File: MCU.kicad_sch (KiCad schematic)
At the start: 36 parts

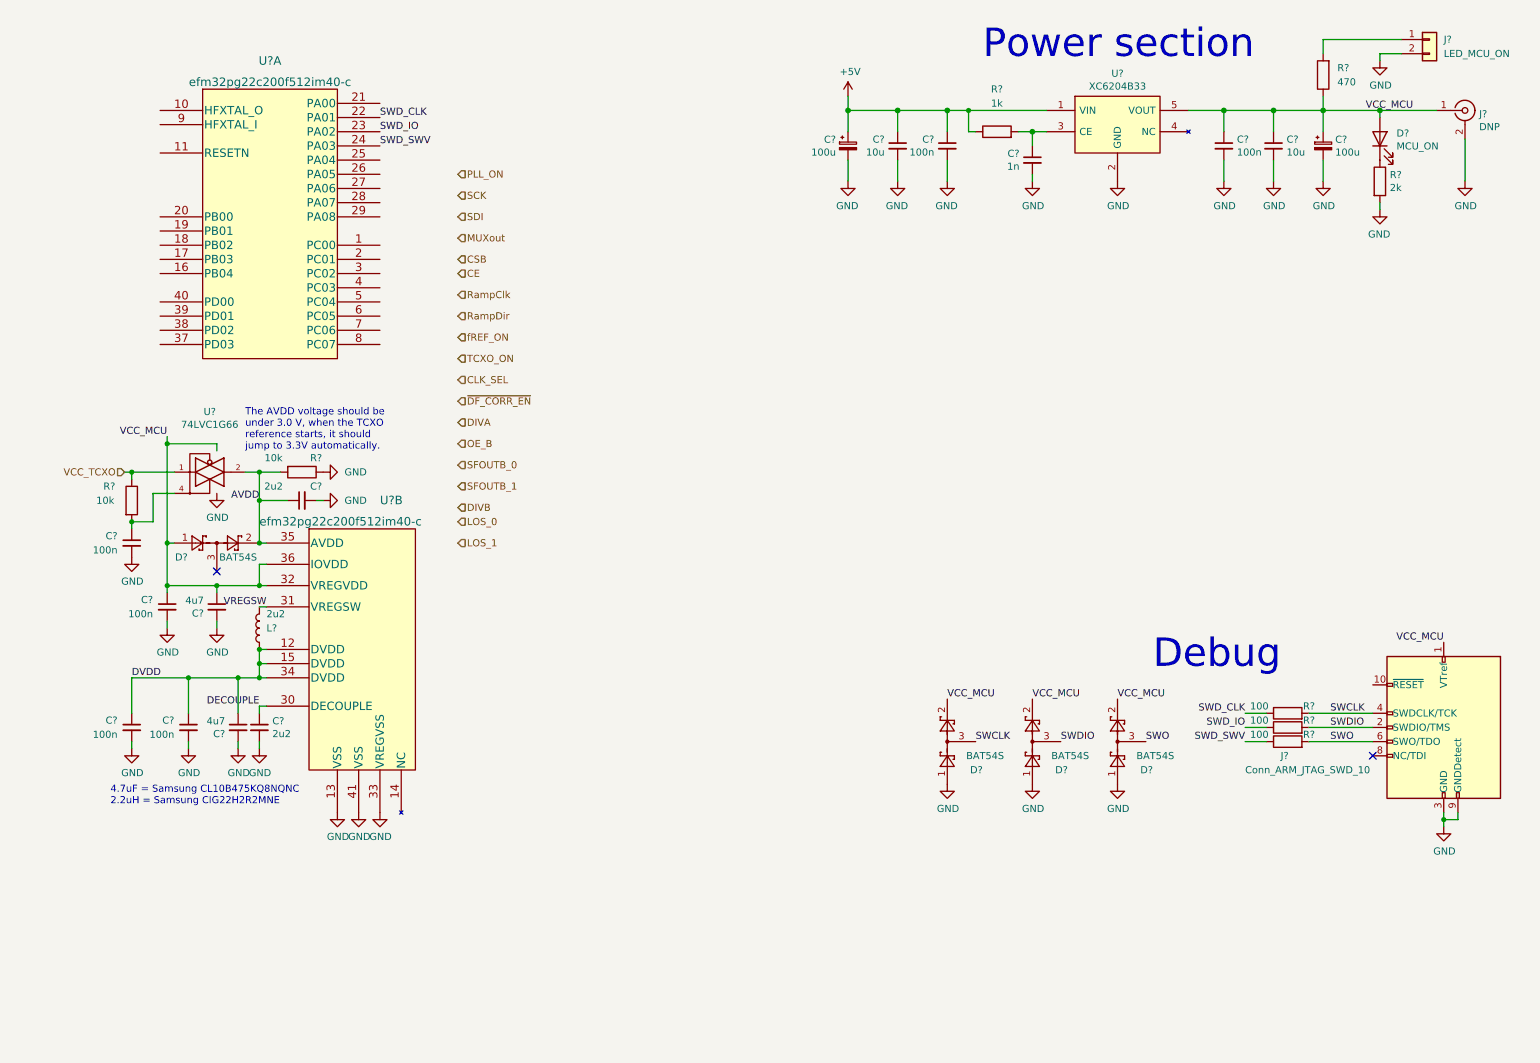
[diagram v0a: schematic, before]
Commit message: Updates to schematic
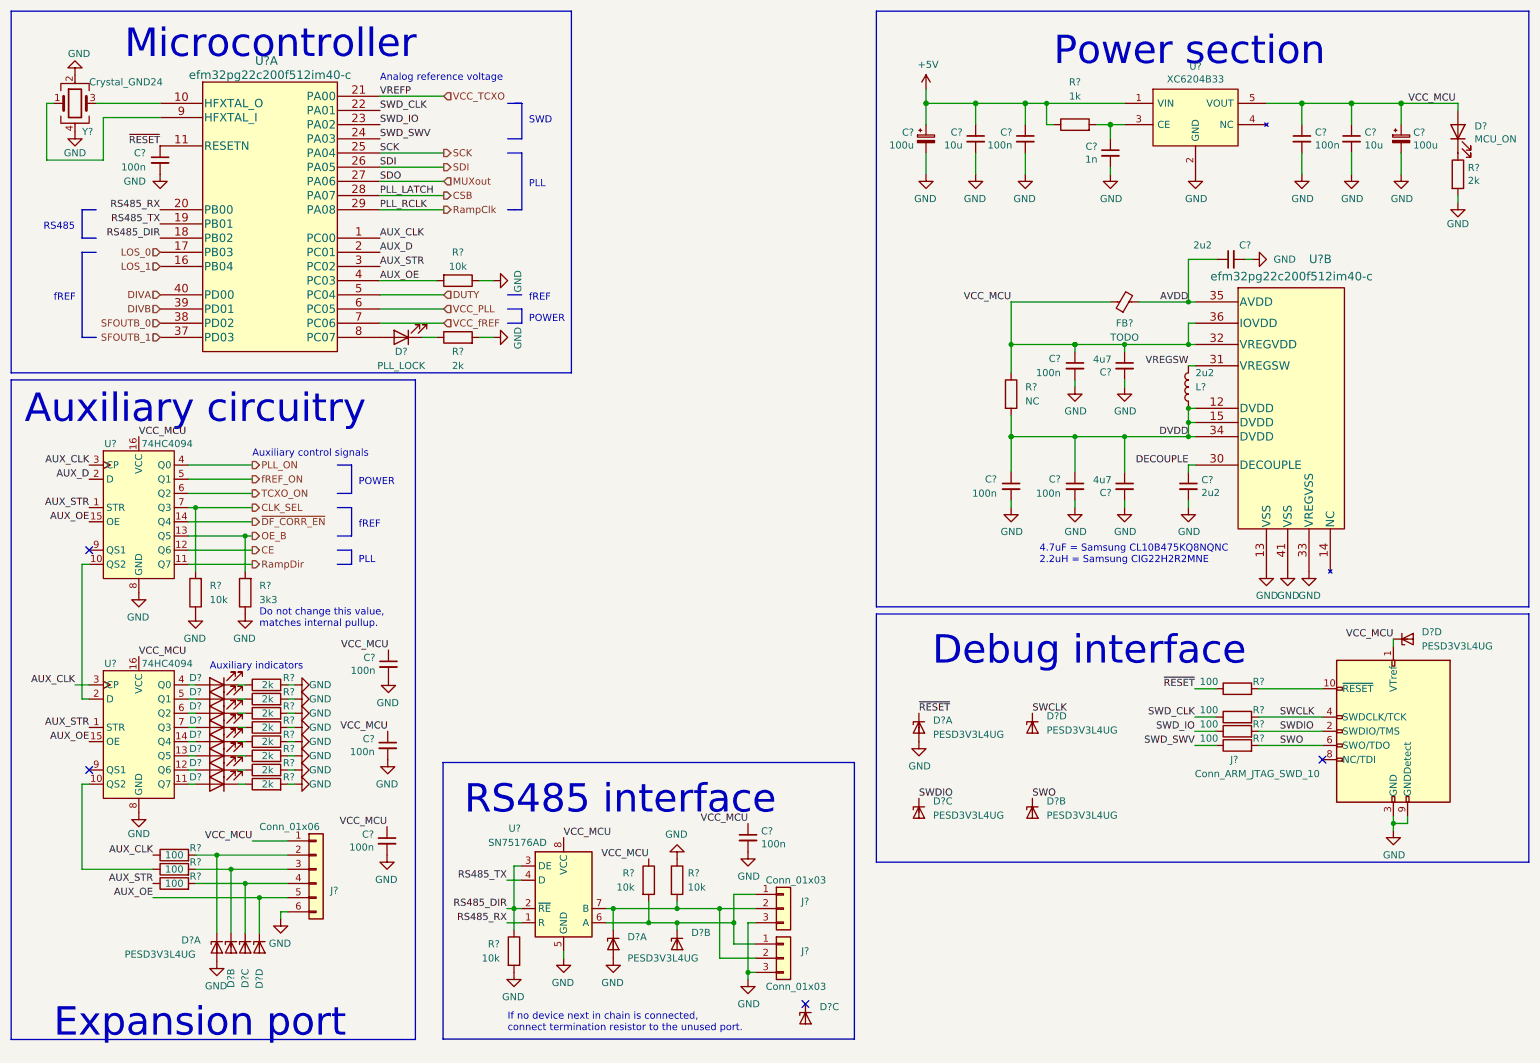
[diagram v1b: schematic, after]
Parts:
- removed C?: 100n, Capacitor_SMD:C_0603_1608Metric_Pad1.08x0.95mm_HandSolder, symbol Device:C_Small
- removed D? (x4): BAT54S, Package_TO_SOT_SMD:SOT-23, symbol Diode:BAT54S
- removed J?: LED_MCU_ON, symbol Connector_Generic:Conn_01x02
- removed J?: DNP, Connector_Coaxial:U.FL_Molex_MCRF_73412-0110_Vertical, symbol Connector:Conn_Coaxial
- removed R?: 470, Resistor_SMD:R_0603_1608Metric_Pad0.98x0.95mm_HandSolder, symbol Device:R
- removed R? (x2): 10k, Resistor_SMD:R_0603_1608Metric_Pad0.98x0.95mm_HandSolder, symbol Device:R
- removed U?: 74LVC1G66, Package_TO_SOT_SMD:SOT-353_SC-70-5_Handsoldering, symbol 74xGxx:74LVC1G66
- added C? (x5): 100n, Capacitor_SMD:C_0603_1608Metric_Pad1.08x0.95mm_HandSolder, symbol Device:C_Small
- added D?: PLL_LOCK, LED_SMD:LED_0603_1608Metric_Pad1.05x0.95mm_HandSolder, symbol Device:LED
- added D? (x8): (no value), LED_SMD:LED_0603_1608Metric_Pad1.05x0.95mm_HandSolder, symbol Device:LED
- added D? (x12): PESD3V3L4UG, Package_TO_SOT_SMD:SOT-353_SC-70-5, symbol Power_Protection:PESD3V3L4UG
- added FB?: TODO, symbol Device:FerriteBead_Small
- added J? (x2): Conn_01x03, symbol Connector_Generic:Conn_01x03
- added J?: Conn_01x06, symbol Connector_Generic:Conn_01x06
- added R? (x4): 100, Resistor_SMD:R_0603_1608Metric_Pad0.98x0.95mm_HandSolder, symbol Device:R
- added R? (x9): 2k, Resistor_SMD:R_0603_1608Metric_Pad0.98x0.95mm_HandSolder, symbol Device:R
- added R? (x5): 10k, Resistor_SMD:R_0603_1608Metric_Pad0.98x0.95mm_HandSolder, symbol Device:R
- added R?: 3k3, Resistor_SMD:R_0603_1608Metric_Pad0.98x0.95mm_HandSolder, symbol Device:R
- added R?: NC, Resistor_SMD:R_0603_1608Metric_Pad0.98x0.95mm_HandSolder, symbol Device:R
- added U? (x2): 74HC4094, Package_SO:SO-16_3.9x9.9mm_P1.27mm, symbol petr:74HC4094
- added U?: SN75176AD, Package_SO:SOIC-8_3.9x4.9mm_P1.27mm, symbol Interface_UART:SN75176AD
- added Y?: Crystal_GND24, symbol Device:Crystal_GND24
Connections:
- net AVDD: now also FB?.2
- net CE: now also U?.12 (Q6)
- net CLK_SEL: now also R?.2, U?.7 (Q3)
- net CSB: now also U?.28 (PA07)
- net DIVA: now also U?.40 (PD00)
- net DIVB: now also U?.39 (PD01)
- net GND: now also C?.2, C?.2, C?.2, C?.2, C?.2, D?.2 (A), D?.2 (A), D?.2 (A), J?.3 (Pin_3), J?.3 (Pin_3), J?.6 (Pin_6), R?.1, R?.1, R?.1, R?.1, R?.2, R?.2, R?.2, R?.2, R?.2, R?.2, R?.2, R?.2, R?.2, R?.2, U?.5 (GND), U?.8 (GND), U?.8 (GND), Y?.2, Y?.4
- net LOS_0: now also U?.17 (PB03)
- net LOS_1: now also U?.16 (PB04)
- net MUXout: now also U?.27 (PA06)
- net OE_B: now also R?.2, U?.13 (Q5)
- net PLL_ON: now also U?.4 (Q0)
- net RampClk: now also U?.29 (PA08)
- net RampDir: now also U?.11 (Q7)
- net SCK: now also U?.25 (PA04)
- net SDI: now also U?.26 (PA05)
- net SFOUTB_0: now also U?.38 (PD02)
- net SFOUTB_1: now also U?.37 (PD03)
- net SWCLK: now also D?.5 (K4)
- net SWDIO: now also D?.4 (K3)
- net SWO: now also D?.3 (K2)
- net TCXO_ON: now also U?.6 (Q2)
- net VCC_TCXO: now also U?.21 (PA00)
- net fREF_ON: now also U?.5 (Q1)
- net ~{DF_CORR_EN}: now also U?.14 (Q4)
- net AUX_CLK: now reaches U?.1 (PC00)
- net AUX_CLK: now also R?.1, U?.3 (CP), U?.3 (CP)
- net at U?.10 (HFXTAL_O): now also Y?.3
- net ~{RESET}: now reaches U?.11 (RESETN)
- net ~{RESET}: now also C?.1, D?.1 (K1), R?.1
- net RS485_DIR: now reaches U?.18 (PB02)
- net RS485_DIR: now also R?.1, U?.2 (~{RE}), U?.3 (DE)
- net RS485_TX: now reaches U?.19 (PB01)
- net RS485_TX: now also U?.4 (D)
- net AUX_D: now reaches U?.2 (PC01)
- net AUX_D: now also U?.2 (D)
- net RS485_RX: now reaches U?.20 (PB00)
- net RS485_RX: now also U?.1 (R)
- net AUX_STR: now reaches U?.3 (PC02)
- net AUX_STR: now also R?.1, U?.1 (STR), U?.1 (STR)
- net AUX_OE: now reaches U?.4 (PC03)
- net AUX_OE: now also D?.5 (K4), J?.5 (Pin_5), R?.2, U?.15 (OE), U?.15 (OE)
- net DUTY: now reaches U?.5 (PC04)
- net VCC_PLL: now reaches U?.6 (PC05)
- net VCC_fREF: now reaches U?.7 (PC06)
- net at U?.8 (PC07): now also D?.2 (A)
- net at U?.9 (HFXTAL_I): now also Y?.1
- net at J?.10 (~{RESET}): now also R?.2
- net VCC renamed VCC_MCU
- net VCC_MCU: now also C?.1, C?.1, C?.1, C?.1, D?.5 (K4), FB?.1, J?.1 (Pin_1), R?.1, R?.1, U?.16 (VCC), U?.16 (VCC), U?.8 (VCC)
- new net: D?.1 (K1), J?.2 (Pin_2), R?.2
- new net: D?.1 (K), R?.1 (x9)
- new net: R?.1, U?.10 (QS2)
- new net: D?.2 (A), U?.11 (Q7)
- new net: D?.2 (A), U?.12 (Q6)
- new net: D?.2 (A), U?.13 (Q5)
- new net: D?.2 (A), U?.14 (Q4)
- new net: U?.10 (QS2), U?.2 (D)
- new net: D?.2 (A), U?.4 (Q0)
- new net: D?.2 (A), U?.5 (Q1)
- new net: D?.2 (A), U?.6 (Q2)
- new net: D?.2 (A), U?.7 (Q3)
- new net: D?.3 (K2), J?.1 (Pin_1), J?.1 (Pin_1), R?.2, U?.6 (A)
- new net: D?.4 (K3), J?.4 (Pin_4), R?.2
- new net: D?.1 (K1), J?.2 (Pin_2), J?.2 (Pin_2), R?.2, U?.7 (B)
- new net: D?.3 (K2), J?.3 (Pin_3), R?.2
- no-connect marks 2 -> 4
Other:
- note added: "Analog reference voltage"
- note added: "Auxiliary circuitry"
- note added: "Auxiliary control signals"
- note added: "Auxiliary indicators"
- note added: "Debug interface"
- note added: "Do not change this value, matches internal pullup."
- note added: "Expansion port"
- note added: "If no device next in chain is connected, connect termination resistor to the unused port."
- note added: "Microcontroller"
- note added: "PLL"
- note added: "POWER"
- note added: "RS485"
- note added: "RS485 interface"
- note added: "SWD"
- note added: "fREF"
- note removed: "Debug"
- note removed: "The AVDD voltage should be under 3.0 V, when the TCXO reference starts, it should jump to 3.3V automatically."
- moved on the sheet: C?, D?, J?, L?, R?, U?, U?A, U?B
